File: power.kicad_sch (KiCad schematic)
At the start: 39 parts, among them IC1 MP2338GTL-Z, U7 L7805, U8 AMS1117-3.3

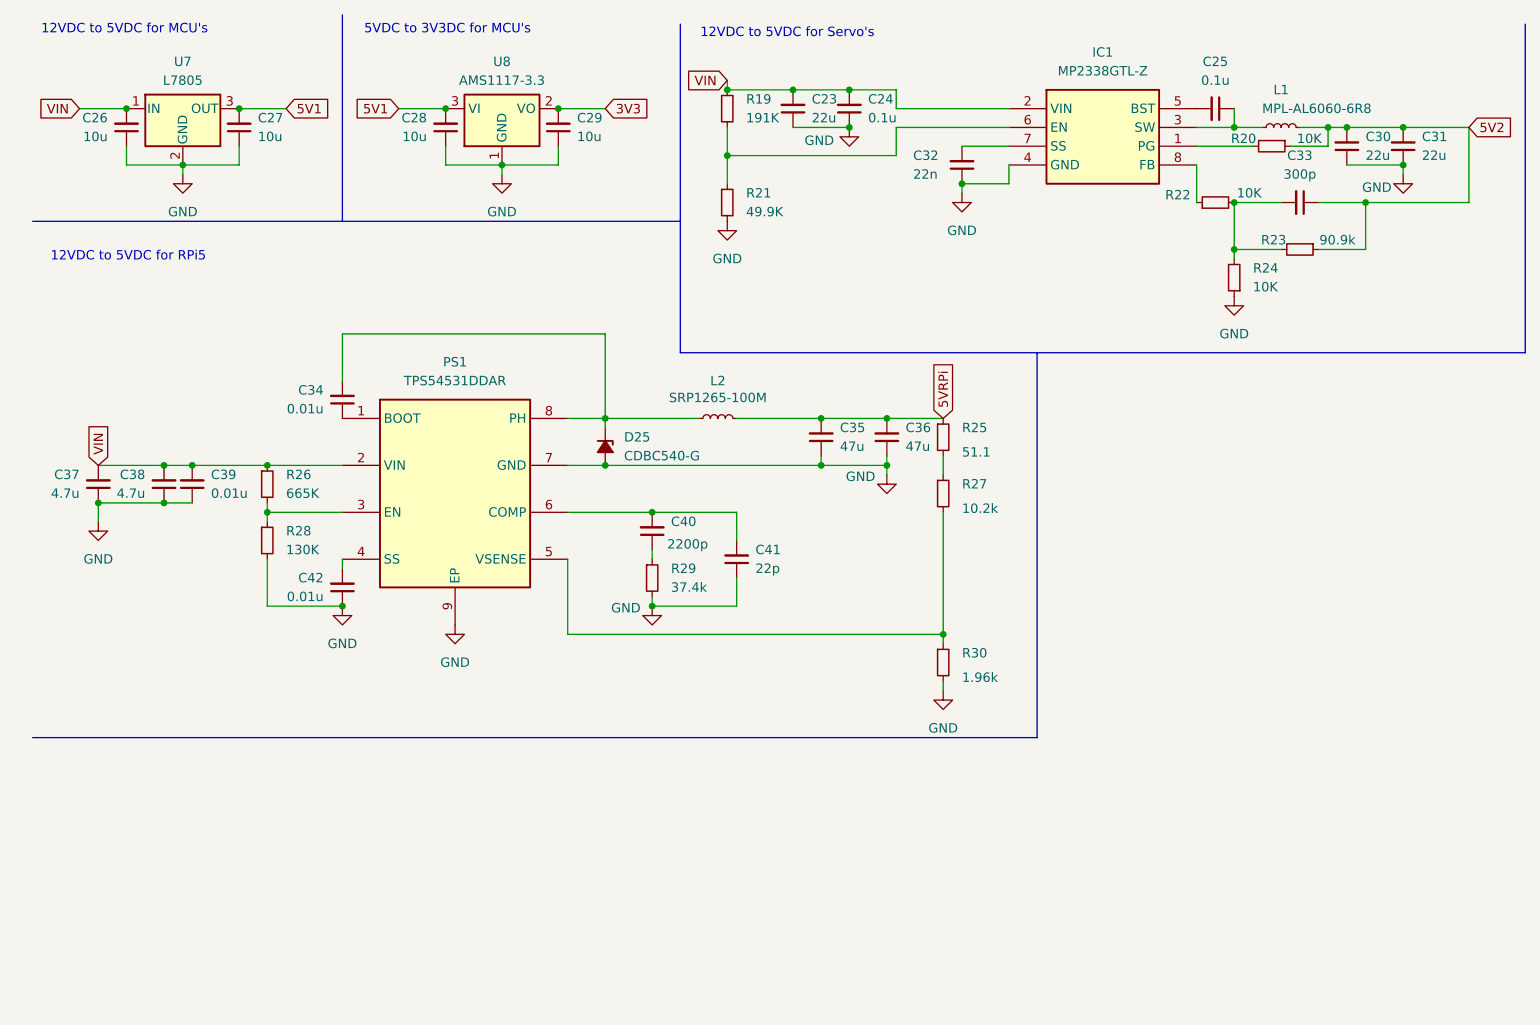
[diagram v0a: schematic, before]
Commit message: Visual Improvements
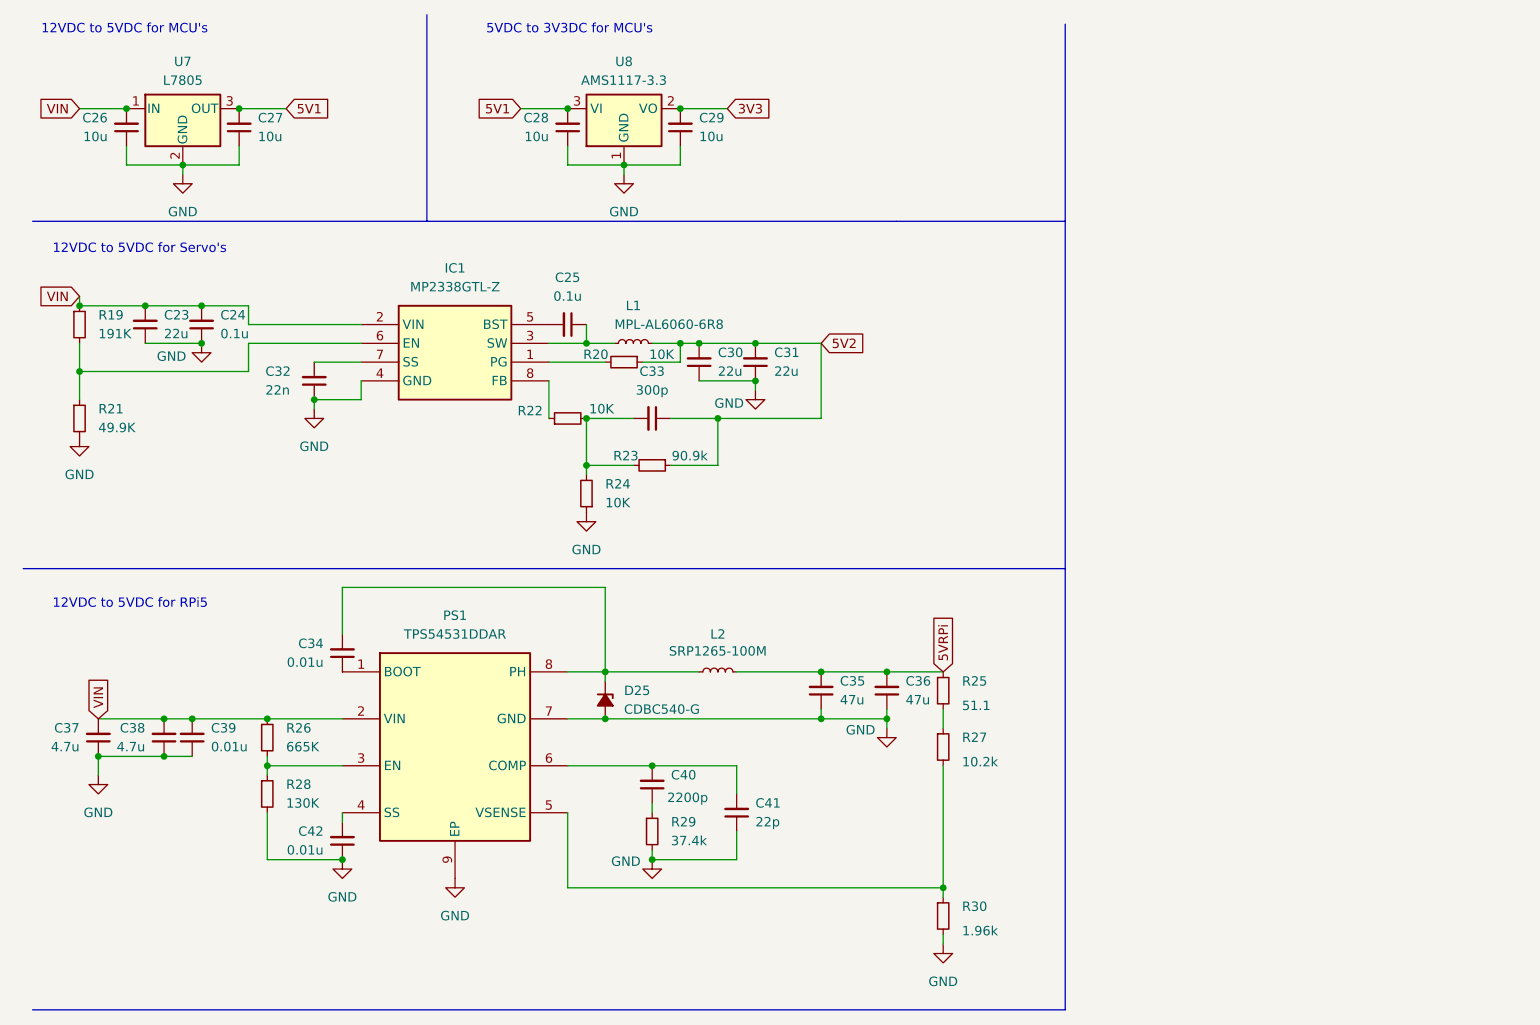
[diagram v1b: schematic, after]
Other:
- moved on the sheet: C23, C24, C25, C28, C29, C30, C31, C32, C33, C34, C35, C36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
